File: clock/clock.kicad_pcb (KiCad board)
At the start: 2 copper layers, 100 x 50 mm, 165 parts, among them J1 Conn_02x05_Odd_Even, P1 Conn_WallPlug, U1 74HC596, U10 74HC596, U11 LPC804-TSSOP24, U2 74HC596, U3 74HC596, U4 74HC596, U5 74HC596, U6 74HC596, U7 L78L33ABU, U8 74HC596, U9 74HC596

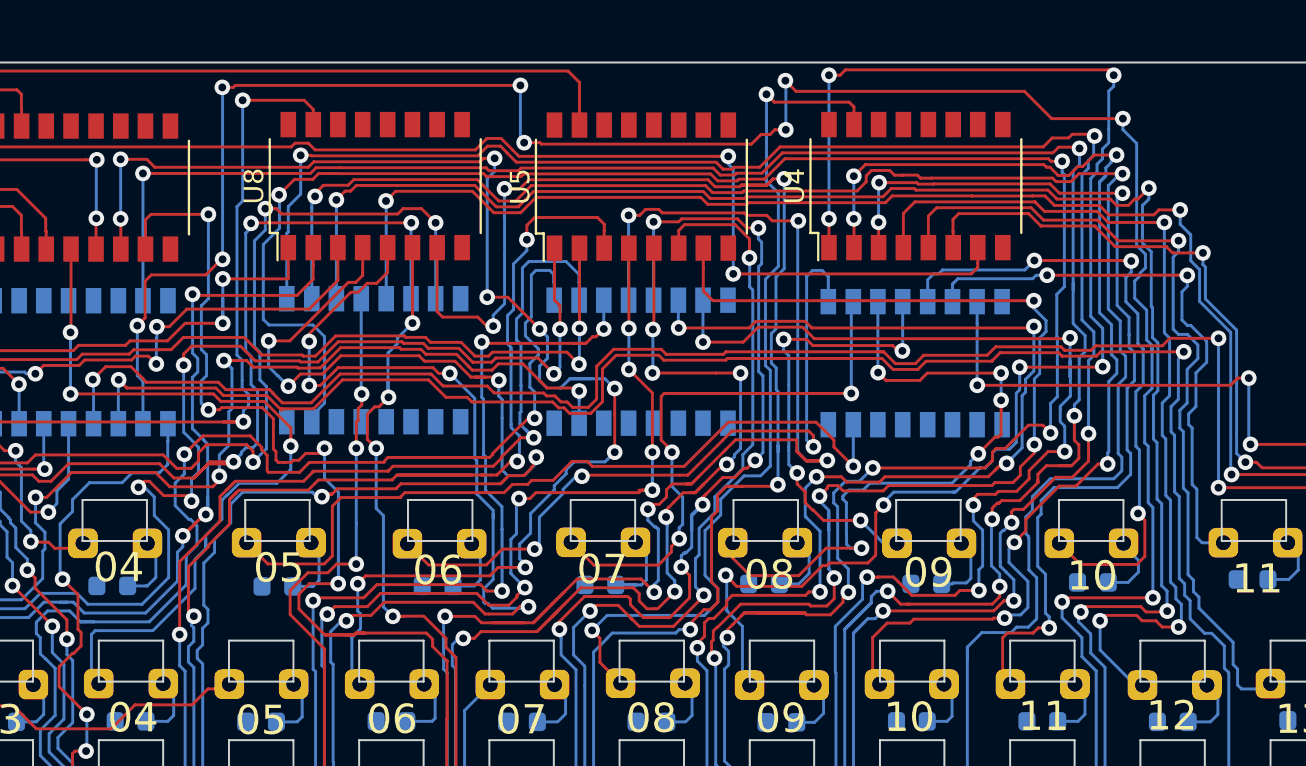
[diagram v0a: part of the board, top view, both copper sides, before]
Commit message: saving progress
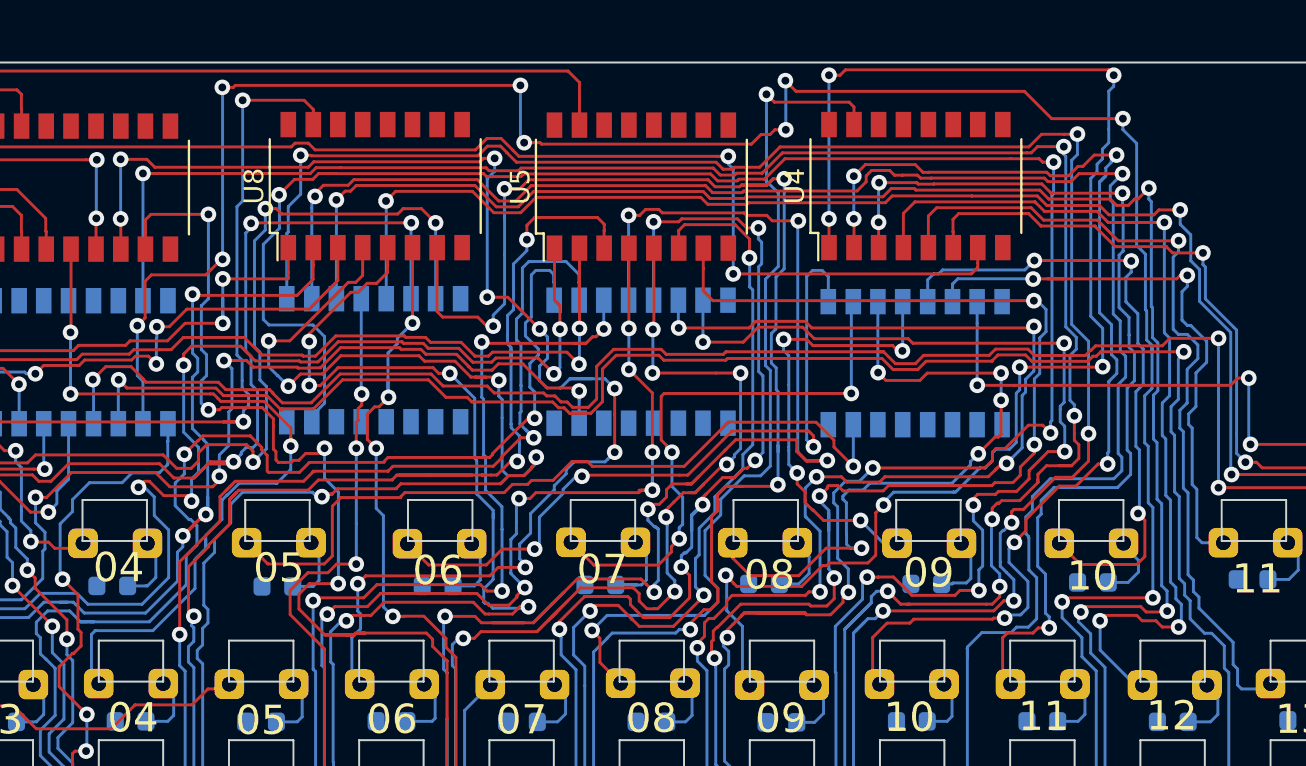
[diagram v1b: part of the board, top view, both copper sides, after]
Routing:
- net M55: track 69.5 -> 68.0 mm
- net M40: track 110.9 -> 109.7 mm
- net M25: track 96.2 -> 95.2 mm
- net H11: track 29.0 -> 29.5 mm
- net M24: track 110.4 -> 109.9 mm
